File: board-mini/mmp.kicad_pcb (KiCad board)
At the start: 2 copper layers, 50 x 15.2 mm, 39 parts, among them IC1 STM32F103C, IC3 SI8662, IC4 MCP1700-33, J1 SWD, P1 USB_B, P2 CONN_01X04, SW1 SW_PUSH, SW3 SW_PUSH, Y1 Crystal_Small

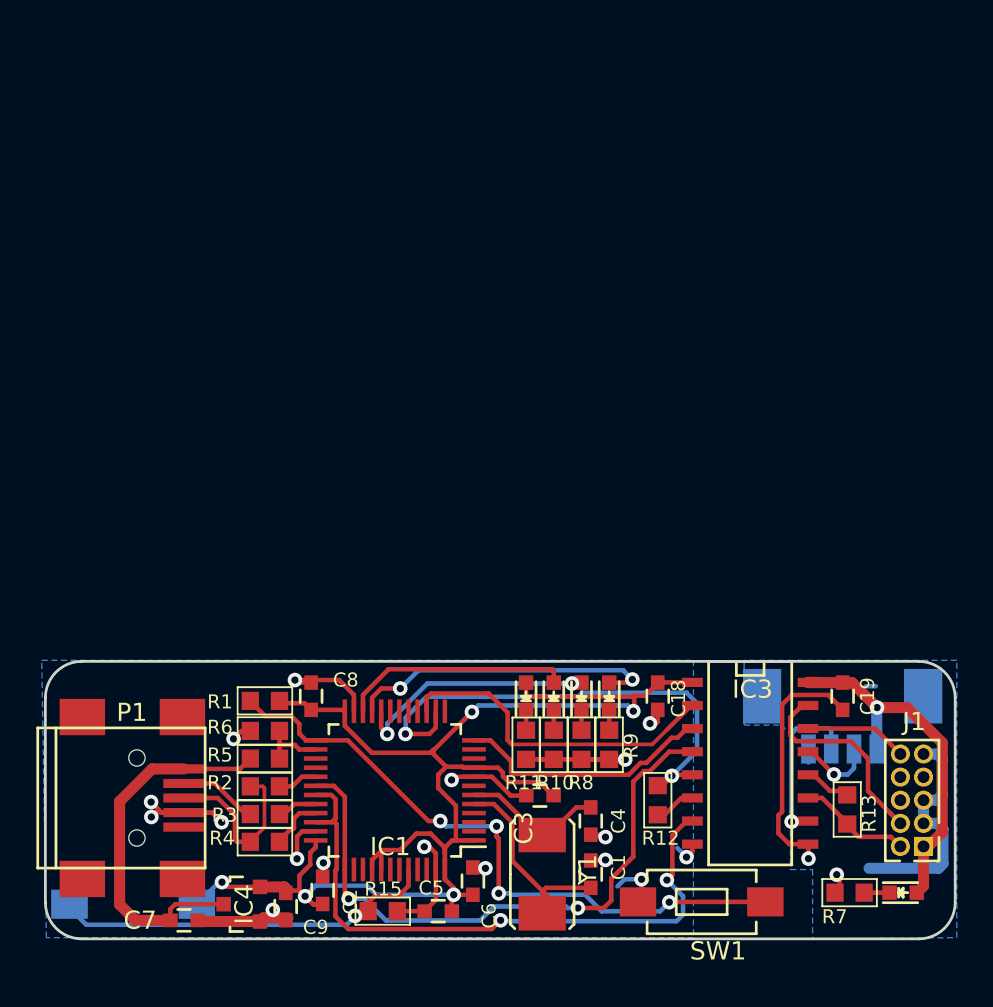
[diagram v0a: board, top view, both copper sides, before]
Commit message: done
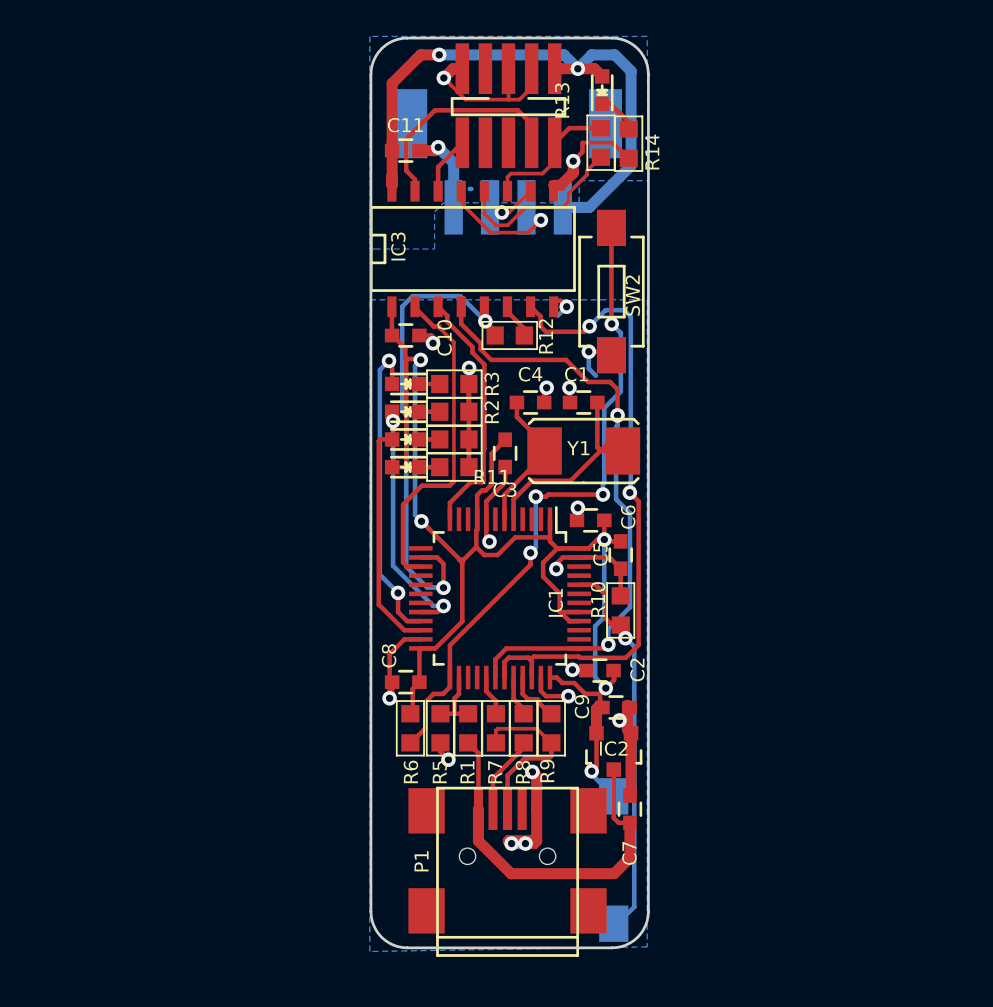
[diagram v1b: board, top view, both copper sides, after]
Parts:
- J1: footprint Pin_Headers:Pin_Header_Straight_2x05_Pitch1.27mm -> agg:FTSH-105-01-L-DV-K
- P2: footprint Connectors_Molex:Connector_Molex_PicoBlade_53261-0471 -> agg:SM04B-PASS
- moved D5 47.1 mm to (208.6, 44.4), turned to 90 degrees
- moved J1 46.7 mm to (203.5, 45.2)
- moved R14 42.9 mm to (210.1, 47.3), turned to 270 degrees
- moved R13 39.1 mm to (208.5, 47.2), turned to 90 degrees
- moved C11 38.4 mm to (197.8, 47.7), turned to 0 degrees
- moved SW2 33.9 mm to (209.1, 55.4), turned to 270 degrees
- moved P2 33.7 mm to (203.4, 49.5), turned to 180 degrees
- moved IC3 32.1 mm to (201.5, 53.1), turned to 0 degrees
- moved R12 26.8 mm to (203.5, 57.8), turned to 0 degrees
- moved SW1 26.5 mm to (209.2, 86.7), turned to 270 degrees
- moved C1 25.9 mm to (207.6, 61.5), turned to 180 degrees
- moved C7 25.3 mm to (210.1, 83.9), turned to 90 degrees
- moved C10 24.2 mm to (197.8, 57.8), turned to 0 degrees
- moved Y1 23.4 mm to (207.6, 64.2), turned to 180 degrees
- moved C4 23.2 mm to (204.7, 61.5), turned to 0 degrees
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- renumbered C18 to C10, C19 to C11, IC4 to IC2, R5 to R1, R15 to R10, R7 to R14, R8 to R2, R9 to R3, R10 to R4, R6 to R5, R1 to R6, R2 to R7, R3 to R8, R4 to R9, SW3 to SW1, SW1 to SW2
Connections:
- P1 pad 4: GND -> Net-(P1-Pad4)
- P1 pad 5: Net-(P1-Pad5) -> GND
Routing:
- net +3.3VP: track 20.5 -> 33.6 mm, vias 1 -> 2
- net GNDREF: track 28.9 -> 20.4 mm, vias 2 -> 3
- net Net-(IC3-Pad12): track 2.28 -> 9.85 mm
- net /Rx: track 9.14 -> 3.24 mm
- net /Tx: track 4.24 -> 7.94 mm
- net Net-(IC3-Pad14): track 5.66 -> 2.88 mm
- net Net-(IC3-Pad11): track 6.41 -> 7.63 mm
- net Net-(D5-Pad1): track 1.19 -> 2.26 mm
- net GND: track 48.2 -> 49.2 mm
- net /H_SWDIO: track 34.8 -> 35.4 mm
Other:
- board size 50 x 15.2 mm -> 15.2 x 50 mm
- board text added: "Feb 2016"
- board text added: "MMP-Isolated"
